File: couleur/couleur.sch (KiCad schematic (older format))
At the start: 15 parts, among them P1 CONN_02X03, P2 Mounting, P3 Mounting, P4 Mounting, P5 Mounting, U1 S4282-51

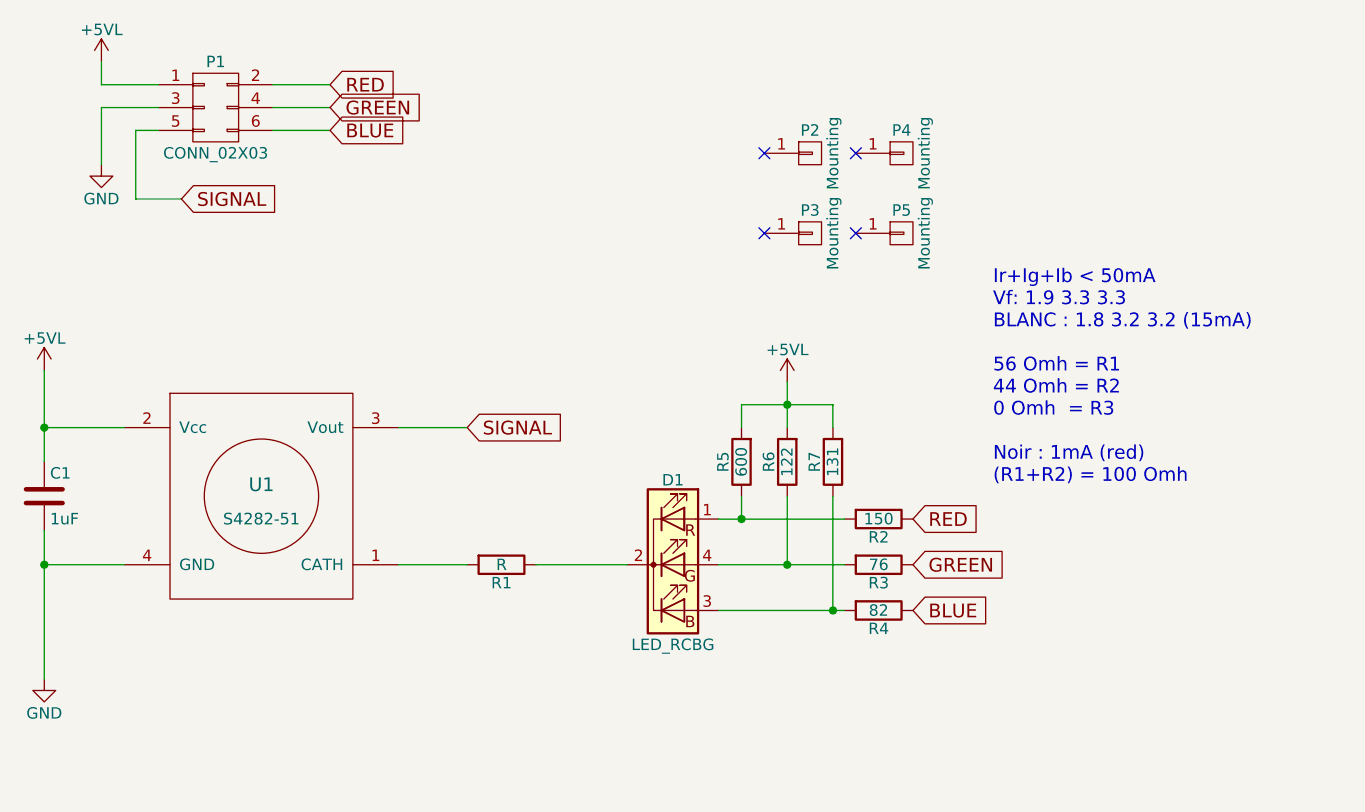
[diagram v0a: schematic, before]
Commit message: Couleur
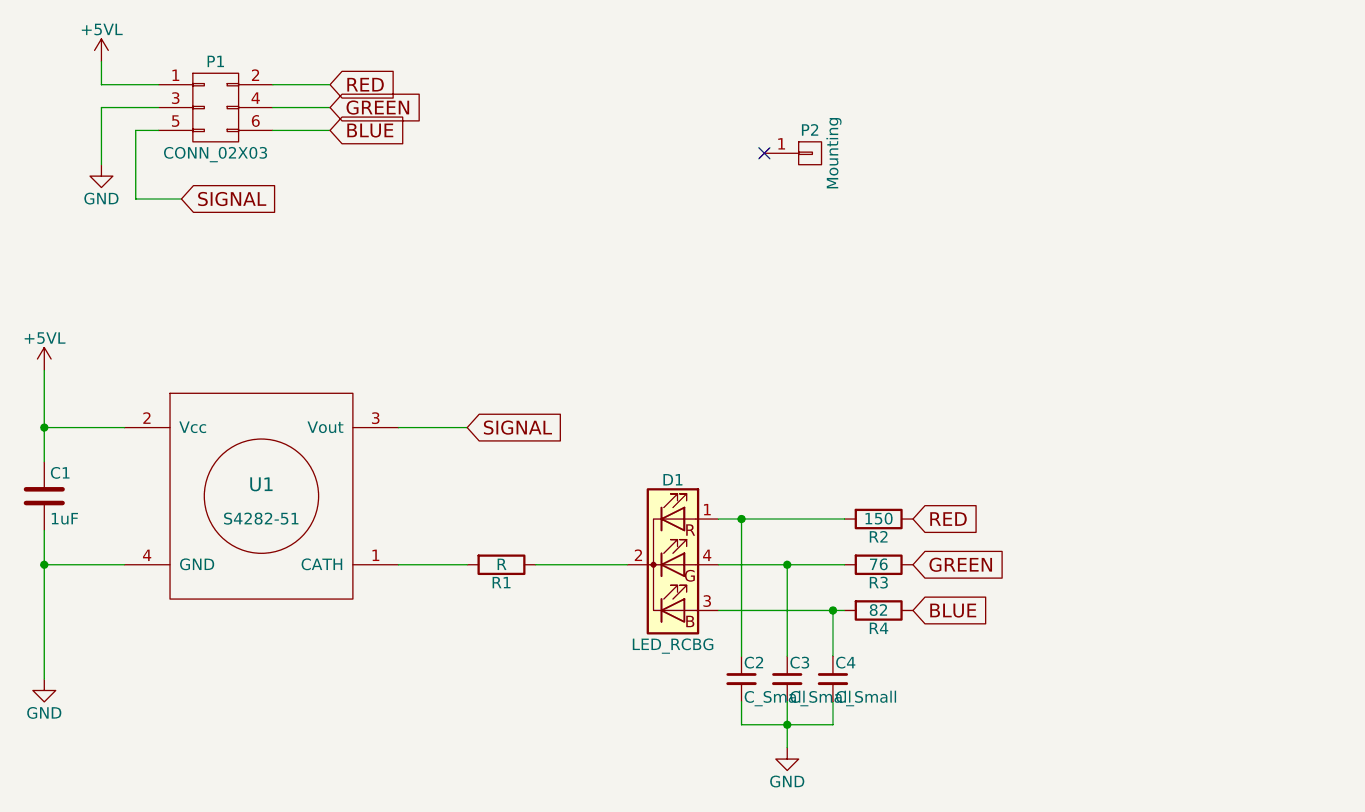
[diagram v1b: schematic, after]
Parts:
- removed P3, P4, P5: Mounting, Mounting_Holes:MountingHole_3.2mm_M3_Pad, symbol CONN_01X01
- removed R5: 600, Resistors_SMD:R_0603_HandSoldering, symbol R
- removed R6: 122, Resistors_SMD:R_0603_HandSoldering, symbol R
- removed R7: 131, Resistors_SMD:R_0603_HandSoldering, symbol R
- added C2, C3, C4: C_Small, Capacitors_SMD:C_0603_HandSoldering, symbol C_Small
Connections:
- net GND: now also C2.2, C3.2, C4.2
- net at D1.1 (RA), R2.2: now also C2.1
- net at D1.4 (GA), R3.2: now also C3.1
- net at D1.3 (BA), R4.2: now also C4.1
- no-connect marks 4 -> 1
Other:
- note removed: "Ir+Ig+Ib < 50mA\nVf: 1.9 3.3 3.3\nBLANC : 1.8 3.2 3.2 (15mA)\n\n56 Omh = R1\n44 Omh = R2\n0 Omh = R3\n\nNoir : 1mA (red)\n(R1+R2) = 100 Omh\n"
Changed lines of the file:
@@
 $EndComp
 $Comp
-L GND #PWR2
+L GND #PWR01
 U 1 1 5A77312B
 P 3550 4800
-F 0 "#PWR2" H 3550 4550 50  0001 C CNN
+F 0 "#PWR01" H 3550 4550 50  0001 C CNN
 F 1 "GND" H 3550 4650 50  0000 C CNN
 F 2 "" H 3550 4800 50  0000 C CNN
@@
 $EndComp
 $Comp
-L +5VL #PWR1
+L +5VL #PWR02
 U 1 1 5A773143
 P 3550 3450
-F 0 "#PWR1" H 3550 3300 50  0001 C CNN
+F 0 "#PWR02" H 3550 3300 50  0001 C CNN
 F 1 "+5VL" H 3550 3590 50  0000 C CNN
 F 2 "" H 3550 3450 50  0000 C CNN
@@
 	3550 4150 3550 4800
 $Comp
-L +5VL #PWR3
+L +5VL #PWR03
 U 1 1 5A773165
 P 3800 2100
-F 0 "#PWR3" H 3800 1950 50  0001 C CNN
+F 0 "#PWR03" H 3800 1950 50  0001 C CNN
 F 1 "+5VL" H 3800 2240 50  0000 C CNN
 F 2 "" H 3800 2100 50  0000 C CNN
@@
 $EndComp
 $Comp
-L GND #PWR4
+L GND #PWR04
 U 1 1 5A773176
 P 3800 2550
-F 0 "#PWR4" H 3800 2300 50  0001 C CNN
+F 0 "#PWR04" H 3800 2300 50  0001 C CNN
 F 1 "GND" H 3800 2400 50  0000 C CNN
 F 2 "" H 3800 2550 50  0000 C CNN
@@
 NoConn ~ 6700 2500
 $Comp
-L CONN_01X01 P3
-U 1 1 5A7B0BC5
-P 6900 2850
-F 0 "P3" H 6900 2950 50  0000 C CNN
-F 1 "Mounting" V 7000 2850 50  0000 C CNN
-F 2 "Mounting_Holes:MountingHole_3.2mm_M3_Pad" H 6900 2850 50  0001 C CNN
-F 3 "" H 6900 2850 50  0000 C CNN
-	1    6900 2850
-	1    0    0    -1
-$EndComp
-NoConn ~ 6700 2850
-$Comp
-L CONN_01X01 P4
-U 1 1 5A7B0C29
-P 7300 2500
-F 0 "P4" H 7300 2600 50  0000 C CNN
-F 1 "Mounting" V 7400 2500 50  0000 C CNN
-F 2 "Mounting_Holes:MountingHole_3.2mm_M3_Pad" H 7300 2500 50  0001 C CNN
-F 3 "" H 7300 2500 50  0000 C CNN
-	1    7300 2500
-	1    0    0    -1
-$EndComp
-$Comp
-L CONN_01X01 P5
-U 1 1 5A7B0CFA
-P 7300 2850
-F 0 "P5" H 7300 2950 50  0000 C CNN
-F 1 "Mounting" V 7400 2850 50  0000 C CNN
-F 2 "Mounting_Holes:MountingHole_3.2mm_M3_Pad" H 7300 2850 50  0001 C CNN
-F 3 "" H 7300 2850 50  0000 C CNN
-	1    7300 2850
-	1    0    0    -1
-$EndComp
-NoConn ~ 7100 2500
-NoConn ~ 7100 2850
-$Comp
 L LED_RCBG D1
 U 1 1 5A7B0E12
@@
 	1    0    0    -1
 $EndComp
-Text Notes 7700 3950 0    60   ~ 0
-Ir+Ig+Ib < 50mA\nVf: 1.9 3.3 3.3\nBLANC : 1.8 3.2 3.2 (15mA)\n\n56 Omh = R1\n44 Omh = R2\n0 Omh  = R3\n\nNoir : 1mA (red)\n(R1+R2) = 100 Omh\n
-$Comp
-L +5VL #PWR5
-U 1 1 5A7B1163
-P 6800 3500
-F 0 "#PWR5" H 6800 3350 50  0001 C CNN
-F 1 "+5VL" H 6800 3640 50  0000 C CNN
-F 2 "" H 6800 3500 50  0000 C CNN
-F 3 "" H 6800 3500 50  0000 C CNN
-	1    6800 3500
-	1    0    0    -1
-$EndComp
-$Comp
-L R R5
-U 1 1 5A7B11FA
-P 6600 3850
-F 0 "R5" V 6680 3850 50  0000 C CNN
-F 1 "600" V 6600 3850 50  0000 C CNN
-F 2 "Resistors_SMD:R_0603_HandSoldering" V 6530 3850 50  0001 C CNN
-F 3 "" H 6600 3850 50  0000 C CNN
-	1    6600 3850
-	-1   0    0    1
-$EndComp
-$Comp
-L R R6
-U 1 1 5A7B1269
-P 6800 3850
-F 0 "R6" V 6880 3850 50  0000 C CNN
-F 1 "122" V 6800 3850 50  0000 C CNN
-F 2 "Resistors_SMD:R_0603_HandSoldering" V 6730 3850 50  0001 C CNN
-F 3 "" H 6800 3850 50  0000 C CNN
-	1    6800 3850
-	-1   0    0    1
-$EndComp
-$Comp
-L R R7
-U 1 1 5A7B12B1
-P 7000 3850
-F 0 "R7" V 7080 3850 50  0000 C CNN
-F 1 "131" V 7000 3850 50  0000 C CNN
-F 2 "Resistors_SMD:R_0603_HandSoldering" V 6930 3850 50  0001 C CNN
-F 3 "" H 7000 3850 50  0000 C CNN
-	1    7000 3850
-	-1   0    0    1
-$EndComp
-Wire Wire Line
-	6800 3500 6800 3700
-Wire Wire Line
-	6600 3700 6600 3600
-Wire Wire Line
-	6600 3600 7000 3600
-Connection ~ 6800 3600
-Wire Wire Line
-	7000 3600 7000 3700
-Wire Wire Line
-	6600 4100 6600 4000
-Wire Wire Line
-	6800 4300 6800 4000
-Wire Wire Line
-	7000 4500 7000 4000
 Connection ~ 6600 4100
 Connection ~ 6800 4300
 Connection ~ 7000 4500
+$Comp
+L C_Small C2
+U 1 1 5A89F2CC
+P 6600 4800
+F 0 "C2" H 6610 4870 50  0000 L CNN
+F 1 "C_Small" H 6610 4720 50  0000 L CNN
+F 2 "Capacitors_SMD:C_0603_HandSoldering" H 6600 4800 50  0001 C CNN
+F 3 "" H 6600 4800 50  0000 C CNN
+	1    6600 4800
+	1    0    0    -1
+$EndComp
+$Comp
+L C_Small C3
+U 1 1 5A89F333
+P 6800 4800
+F 0 "C3" H 6810 4870 50  0000 L CNN
+F 1 "C_Small" H 6810 4720 50  0000 L CNN
+F 2 "Capacitors_SMD:C_0603_HandSoldering" H 6800 4800 50  0001 C CNN
+F 3 "" H 6800 4800 50  0000 C CNN
+	1    6800 4800
+	1    0    0    -1
+$EndComp
+$Comp
+L C_Small C4
+U 1 1 5A89F382
+P 7000 4800
+F 0 "C4" H 7010 4870 50  0000 L CNN
+F 1 "C_Small" H 7010 4720 50  0000 L CNN
+F 2 "Capacitors_SMD:C_0603_HandSoldering" H 7000 4800 50  0001 C CNN
+F 3 "" H 7000 4800 50  0000 C CNN
+	1    7000 4800
+	1    0    0    -1
+$EndComp
+Wire Wire Line
+	6600 4100 6600 4700
+Wire Wire Line
+	6800 4300 6800 4700
+Wire Wire Line
+	7000 4500 7000 4700
+$Comp
+L GND #PWR05
+U 1 1 5A89F54A
+P 6800 5100
+F 0 "#PWR05" H 6800 4850 50  0001 C CNN
+F 1 "GND" H 6800 4950 50  0000 C CNN
+F 2 "" H 6800 5100 50  0000 C CNN
+F 3 "" H 6800 5100 50  0000 C CNN
+	1    6800 5100
+	1    0    0    -1
+$EndComp
+Wire Wire Line
+	6600 4900 6600 5000
+Wire Wire Line
+	6600 5000 7000 5000
+Wire Wire Line
+	6800 4900 6800 5100
+Connection ~ 6800 5000
+Wire Wire Line
+	7000 5000 7000 4900
 $EndSCHEMATC
